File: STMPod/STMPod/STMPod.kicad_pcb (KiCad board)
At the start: 2 copper layers, 18 parts, among them J1 Conn_01x04_Male, J2 Conn_01x12_Male, J3 Conn_01x12_Male, J4 USB_B_Mini, SW1 SW_SPST, U1 STM32F030F4Px, U2 MIC2920A-3.3WS, Y1 Resonator

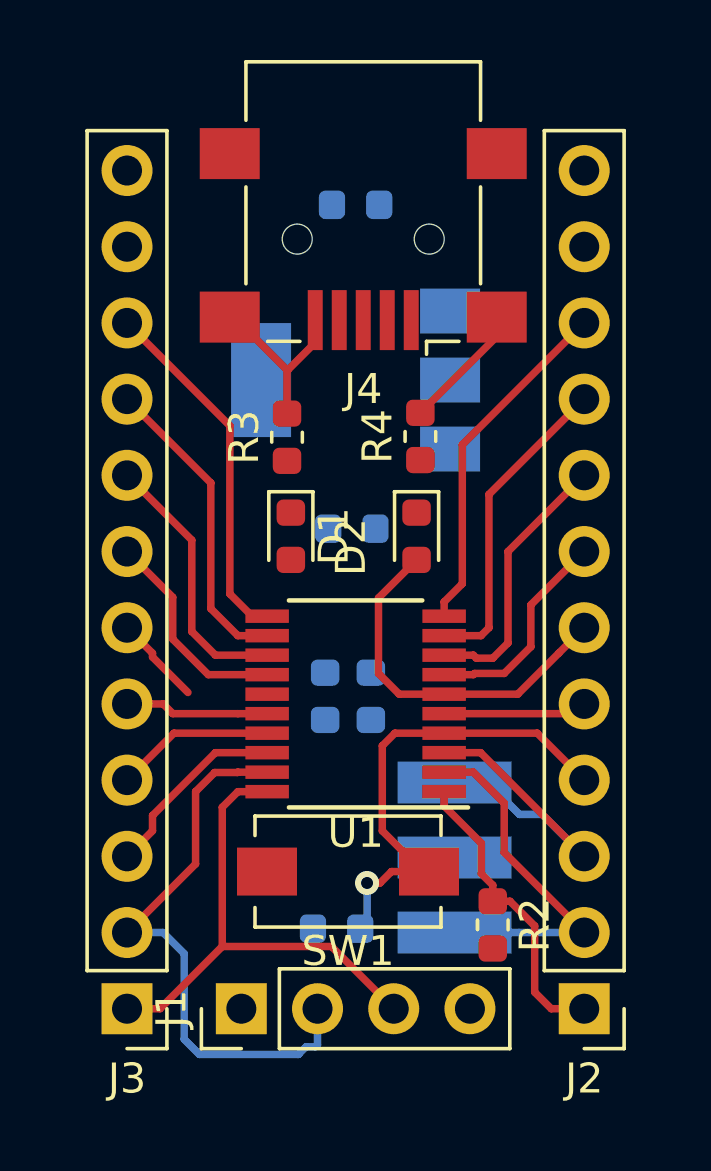
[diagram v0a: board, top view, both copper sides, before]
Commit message: PCB Finished
Done with layout, 3D preview, next step is generating gerbers
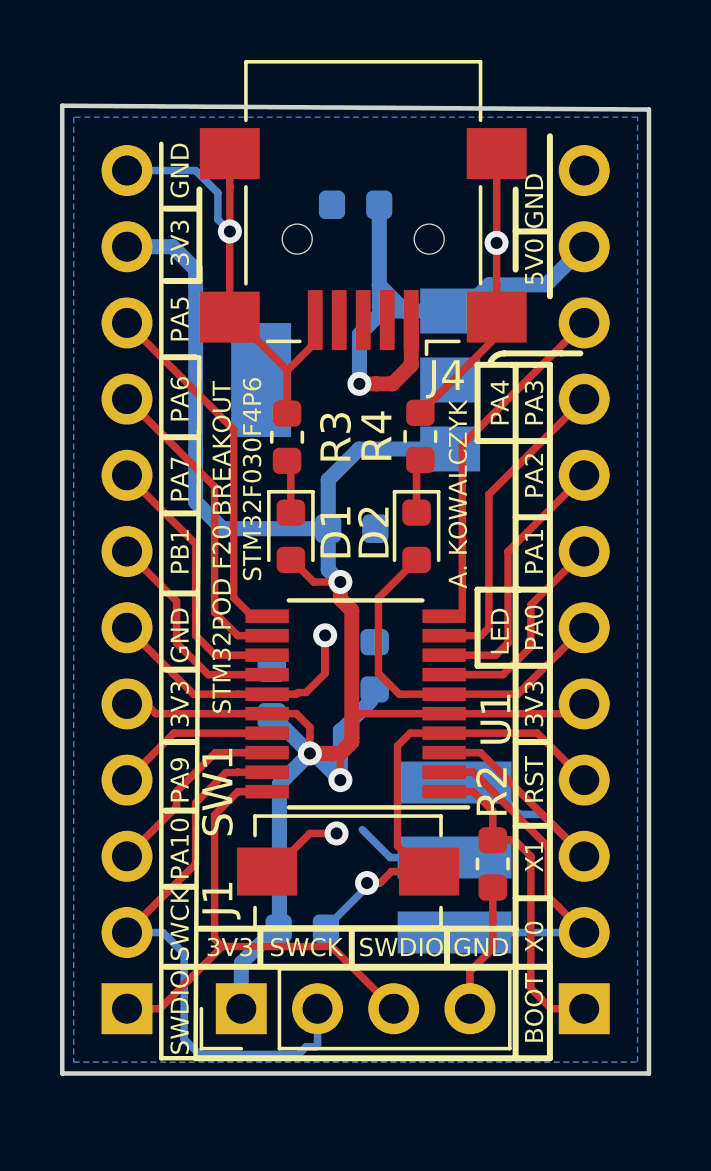
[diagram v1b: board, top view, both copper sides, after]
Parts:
- added REF**: OSHW-Logo2_7.3x6mm_SilkScreen, Symbol:OSHW-Logo2_7.3x6mm_SilkScreen, B.Cu at (171.7, 94.6)
- J2, J3: moved to B.Cu
- moved R2 2.03 mm to (179.8, 96.8)
- moved C3 1.78 mm to (172.5, 91.1)
- moved R1 1.14 mm to (173.5, 98.9)
- moved C4 1.02 mm to (175.9, 90.2)
- turned C1 to 180 degrees
- turned J2 to 0 degrees
- turned J3 to 0 degrees
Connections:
- J3 pad 6: /GND -> GNDREF
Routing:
- net +3V3: track 9.61 -> 66.7 mm, vias 0 -> 3
- net GNDREF: track 10.4 -> 47.1 mm, vias 0 -> 4
- net +5V: track 0.00 -> 20.9 mm, vias 0 -> 1
- net /GND: track 3.00 -> 0.00 mm
- net Net-(D2-Pad1): track 0.00 -> 1.81 mm
- net Net-(D1-Pad1): track 0.00 -> 1.78 mm
- net /BOOT: track 10.2 -> 11.4 mm
- added copper zone on B.Cu, net GNDREF
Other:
- board outline added: 19.6 x 32.3 mm
- board text added: "3V3"
- board text added: "5V0"
- board text added: "A. KOWALCZYK"
- board text added: "BOOT"
- board text added: "GND"
- board text added: "LED"
- board text added: "PA0"
- board text added: "PA1"
- board text added: "PA10"
- board text added: "PA2"
- board text added: "PA3"
- board text added: "PA4"
- board text added: "PA5"
- board text added: "PA6"
- board text added: "PA7"
- board text added: "PA9"
- board text added: "PB1"
- board text added: "RST"
- board text added: "STM32F030F4P6"
- board text added: "STM32POD F20 BREAKOUT"
- board text added: "SWCK"
- board text added: "SWDIO"
- board text added: "X0"
- board text added: "X1"

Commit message: EFM32 Schematic
Schematic done, layout started
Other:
- rule pad_to_mask_clearance: 0.2 -> 0
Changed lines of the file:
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@@
     (mod_text_size 1 1)
     (mod_text_width 0.15)
-    (pad_size 1.524 1.524)
-    (pad_drill 0.762)
-    (pad_to_mask_clearance 0.2)
+    (pad_size 1.45 0.45)
+    (pad_drill 0)
+    (pad_to_mask_clearance 0)
     (aux_axis_origin 0 0)
     (visible_elements 7FFFFFFF)
